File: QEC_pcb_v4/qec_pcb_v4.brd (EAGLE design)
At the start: 53.6 x 35.6 mm, 6 parts

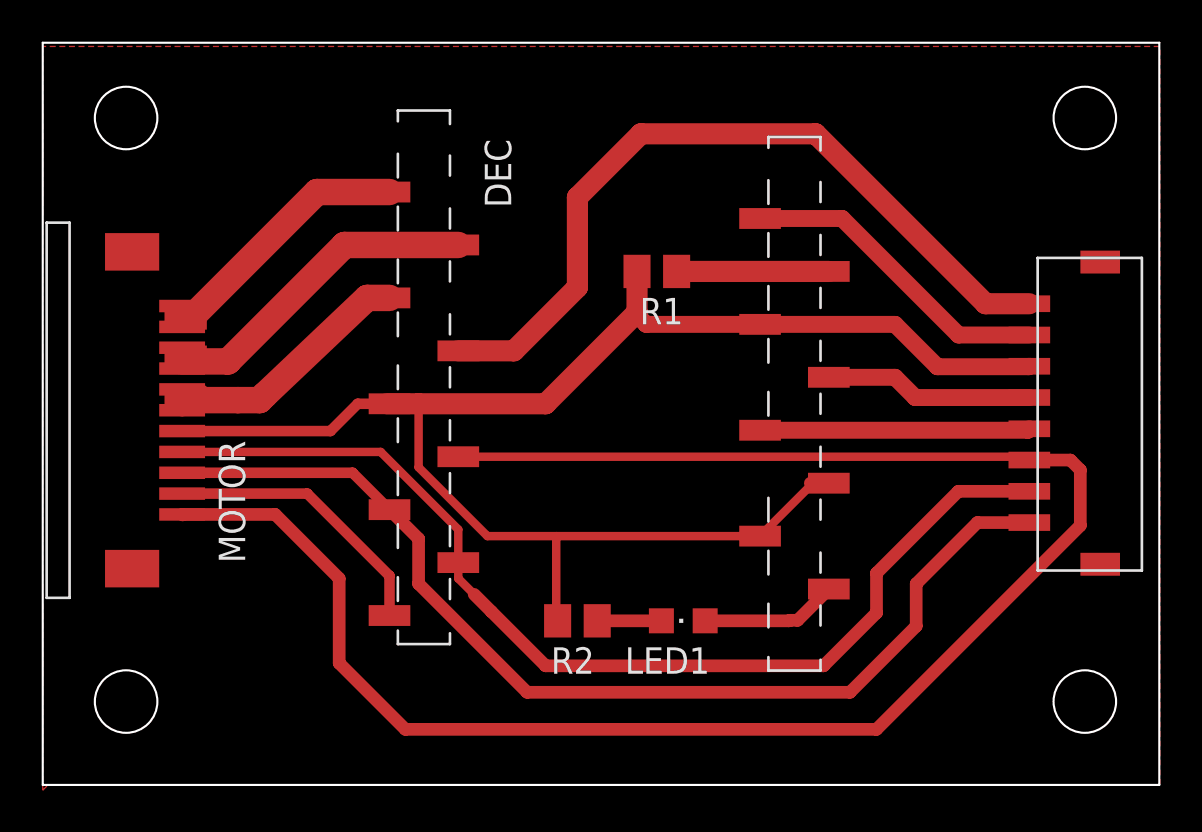
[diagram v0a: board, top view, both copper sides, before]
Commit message: update directories
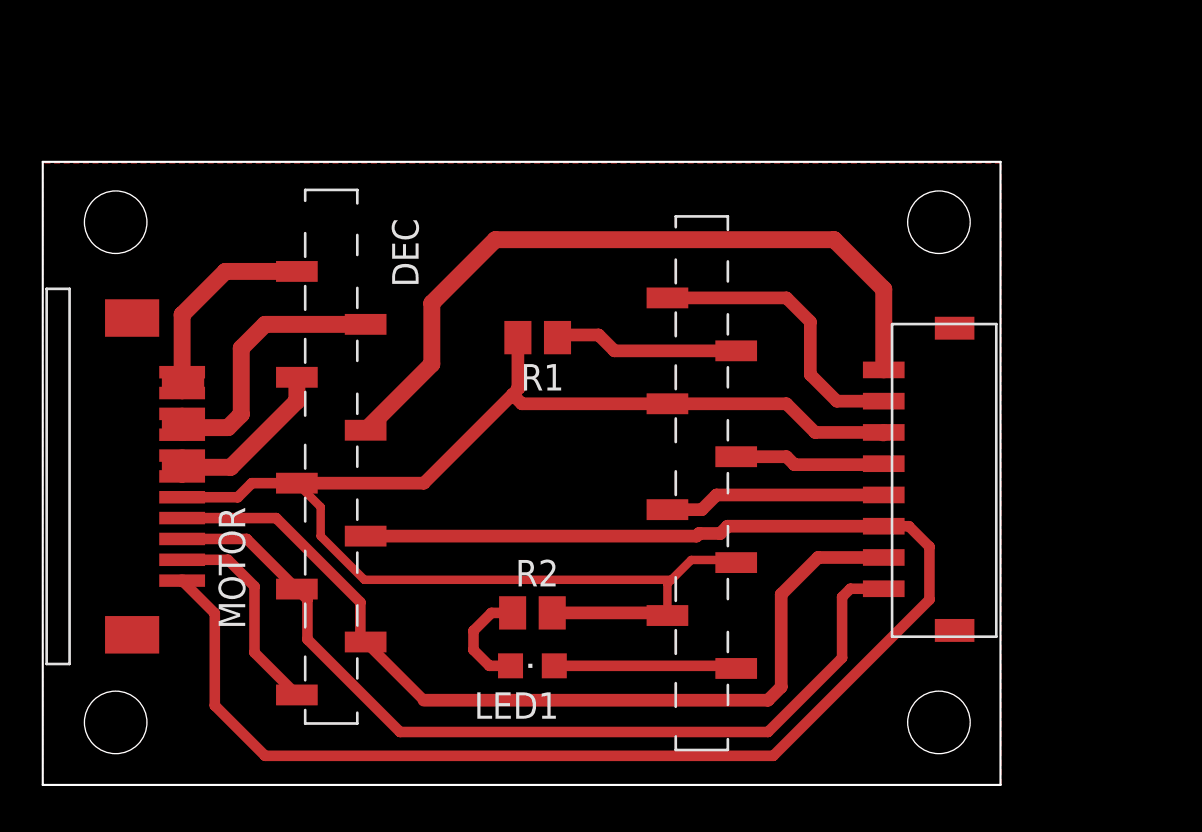
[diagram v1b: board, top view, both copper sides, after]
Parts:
- moved CTRL 7.67 mm to (43.1, 15.1)
- moved LED1 7.55 mm to (23.5, 5.71)
- moved R1 6.54 mm to (23.7, 21.5)
- moved DEC 5.85 mm to (22.7, 17.0)
- moved MOTOR 3.17 mm to (5.59, 11.3)
- moved R2 2.19 mm to (23.5, 8.26), turned to 180 degrees
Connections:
- net N$16 renamed H3
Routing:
- net V+: track 87.0 -> 75.3 mm
- net N$12: track 18.7 -> 9.14 mm
- net N$11: track 22.2 -> 13.7 mm
- net H1: track 51.6 -> 43.2 mm
- net H2: track 52.0 -> 43.7 mm
- net GND: track 78.2 -> 73.2 mm
- net N$5: track 15.1 -> 10.1 mm
- net DIR: track 10.9 -> 7.44 mm
- net H3: track 13.5 -> 10.1 mm
- net +24V: track 37.6 -> 35.2 mm
- net N$2: track 6.56 -> 8.78 mm
- net N$1: track 3.08 -> 5.24 mm
- net EN: track 12.9 -> 10.9 mm
- net N$6: track 7.30 -> 8.94 mm
- net SVS: track 15.2 -> 13.9 mm
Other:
- board size 53.6 x 35.6 mm -> 46 x 29.9 mm
